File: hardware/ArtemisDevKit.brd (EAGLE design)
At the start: 94 x 38.1 mm, 231 parts, among them J1 USB, J10 SMD, J11 SMD, J12 PTH, J14 PTH, J2 CORTEX_JTAG_DEBUG_MINIMUM_PTH, J22 PTH, J23 PTH, J24 PTH, J25 PTH, J26 PTH, J3 CORTEX_JTAG_DEBUG_PTH, J4 SMD, J5 SMD, J6 QWIIC_RIGHT_ANGLE, J7 CAMERA-HIMAX, J8 PTH, J9 SMD, U1 DAPLINK_KL26Z128VFM4, U2 ARTEMIS_MODULESMD, U3 LIS2DH12, U4 AP2127K-1.8V, U5 3.3V, X1 16MHz, Y1 32.768kHz

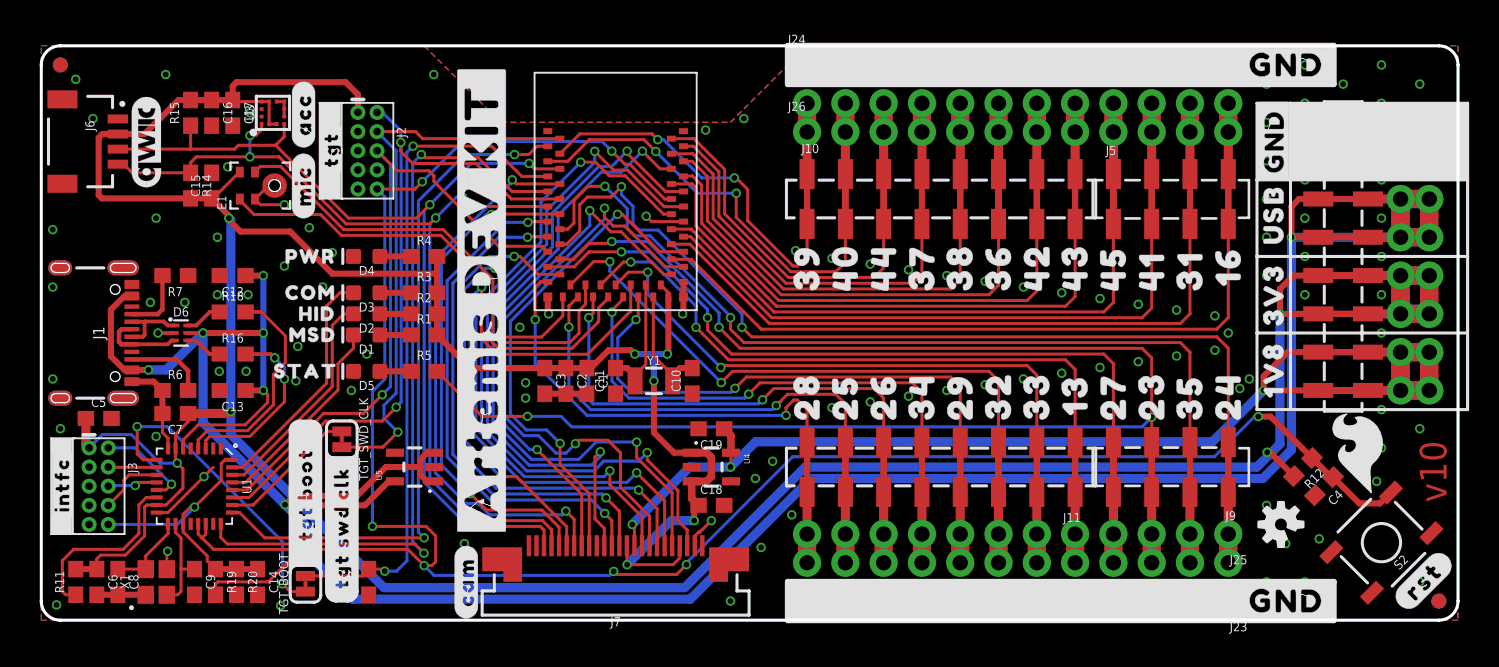
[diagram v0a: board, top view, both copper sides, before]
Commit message: update silkscreen
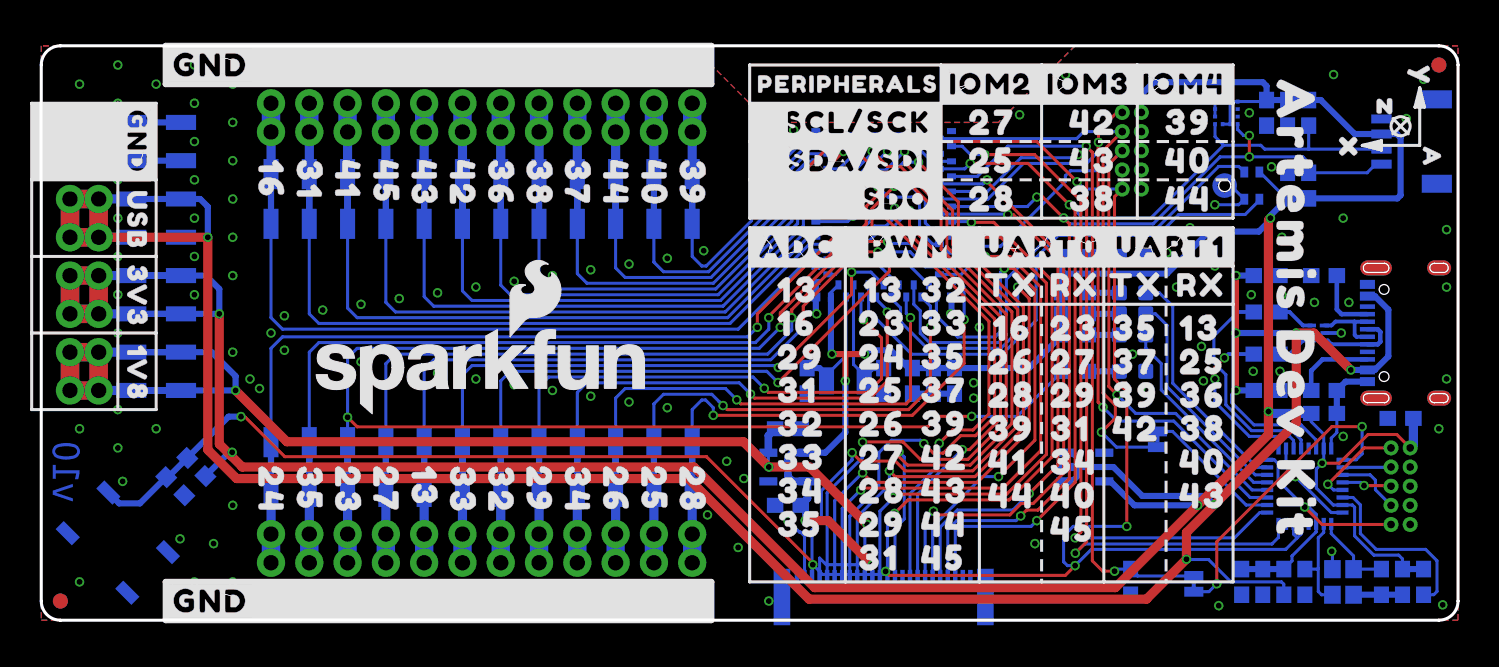
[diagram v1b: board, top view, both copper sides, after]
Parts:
- removed U$143: (no value), SparkFun-Aesthetics:SFE_LOGO_NAME_FLAME_.2
- added LOGO2: SFE_LOGO_NAME_FLAME.2_INCH, SparkFun-Aesthetics:SFE_LOGO_NAME_FLAME_.2
- J5, J9: value SMD -> 1X04_SMD_STRAIGHT_COMBO
- J7: device SparkFun-Connectors:FPC-24-AMPHENOL-SFV24R-1STE1HLF -> SparkFun-Connectors:FPC05024-42201
- U$111: device buzzard_labels:1_#ARTEMIS_DEV_KIT# -> buzzard_labels:#SDA#SDI#24
- U$112: device buzzard_labels:0_#ARTEMIS_DEV_KIT# -> buzzard_labels:#SDO#25
- U$35: device buzzard_labels:22_#SCL#SCLK# -> buzzard_labels:ARTEMIS_DEV_KIT0
- U$36: device buzzard_labels:23_#SDA#MISO# -> buzzard_labels:ARTEMIS_DEV_KIT1
- U$37: device buzzard_labels:24_#MOSI# -> buzzard_labels:#SCL#SCK#23
- moved FD1 91.4 mm to (92.7, 36.8), flipped to the bottom
- moved FD2 91.4 mm to (92.7, 36.8), flipped to the top
- moved FD3 91.4 mm to (1.27, 1.27), flipped to the bottom
- moved FD4 91.4 mm to (1.27, 1.27), flipped to the top
- moved U$135 91.2 mm to (92.6, 6.48), flipped to the bottom
- moved U$113 90.5 mm to (92.2, 30.7), flipped to the top
- moved J8 90.2 mm to (1.91, 33.0), flipped to the bottom
- moved U$115 89.5 mm to (91.8, 36.1), flipped to the top
- moved R11 89.4 mm to (91.7, 2.54), flipped to the bottom
- moved C6 86.6 mm to (90.3, 2.54), flipped to the bottom
- moved C5 86.4 mm to (90.2, 13.4), flipped to the bottom
- moved J12 86.4 mm to (3.81, 33.0), flipped to the bottom
- moved J3 86.4 mm to (90.2, 8.89), flipped to the bottom
- moved U$142 86.2 mm to (3.87, 1.02), flipped to the bottom
- moved C8 83.8 mm to (88.9, 2.54), flipped to the bottom
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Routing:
- net GND: track 109.8 -> 113.0 mm
- net CAMERA_PCLK: track 34.5 -> 36.5 mm
- net SDA: track 65.1 -> 67.1 mm
- net CAMERA_TRIG: track 36.1 -> 38.1 mm
- net CAMERA_INT: track 37.2 -> 39.2 mm
- net 1.8V: track 87.3 -> 89.3 mm
- net CAMERA_VSYNC: track 42.0 -> 44.0 mm
- net CAMERA_HSYNC: track 33.3 -> 35.3 mm
- net CAMERA_D6: track 33.6 -> 35.6 mm
- net CAMERA_D5: track 33.5 -> 35.5 mm
- net CAMERA_D3: track 44.1 -> 46.1 mm
- net CAMERA_D2: track 44.2 -> 46.2 mm
- net CAMERA_D1: track 48.7 -> 50.7 mm
- net CAMERA_MCLK: track 40.1 -> 42.1 mm
- net CAMERA_D7: track 34.3 -> 36.3 mm
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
